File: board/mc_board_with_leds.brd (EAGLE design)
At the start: 131 x 76.6 mm, 30 parts, among them IC2 MEGA8-P, Q2 16MHz

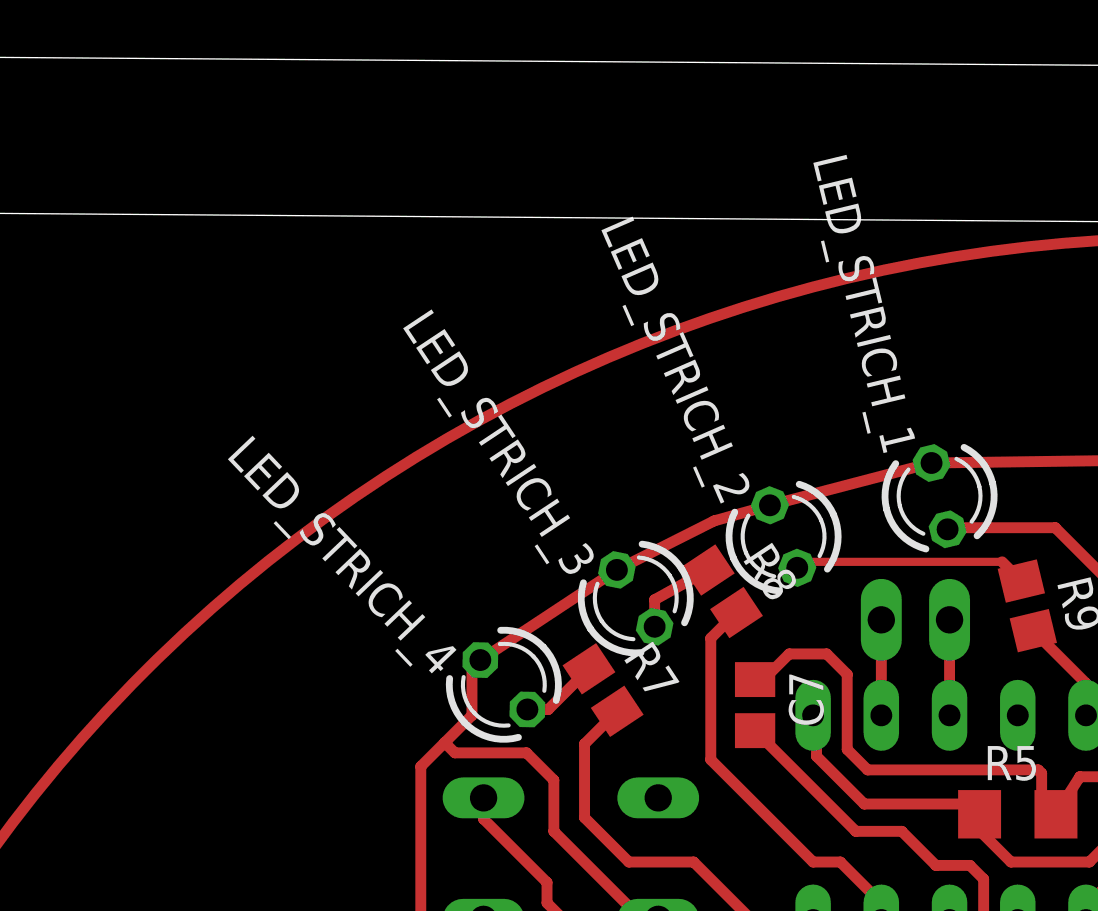
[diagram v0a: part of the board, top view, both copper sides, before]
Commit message: small changes
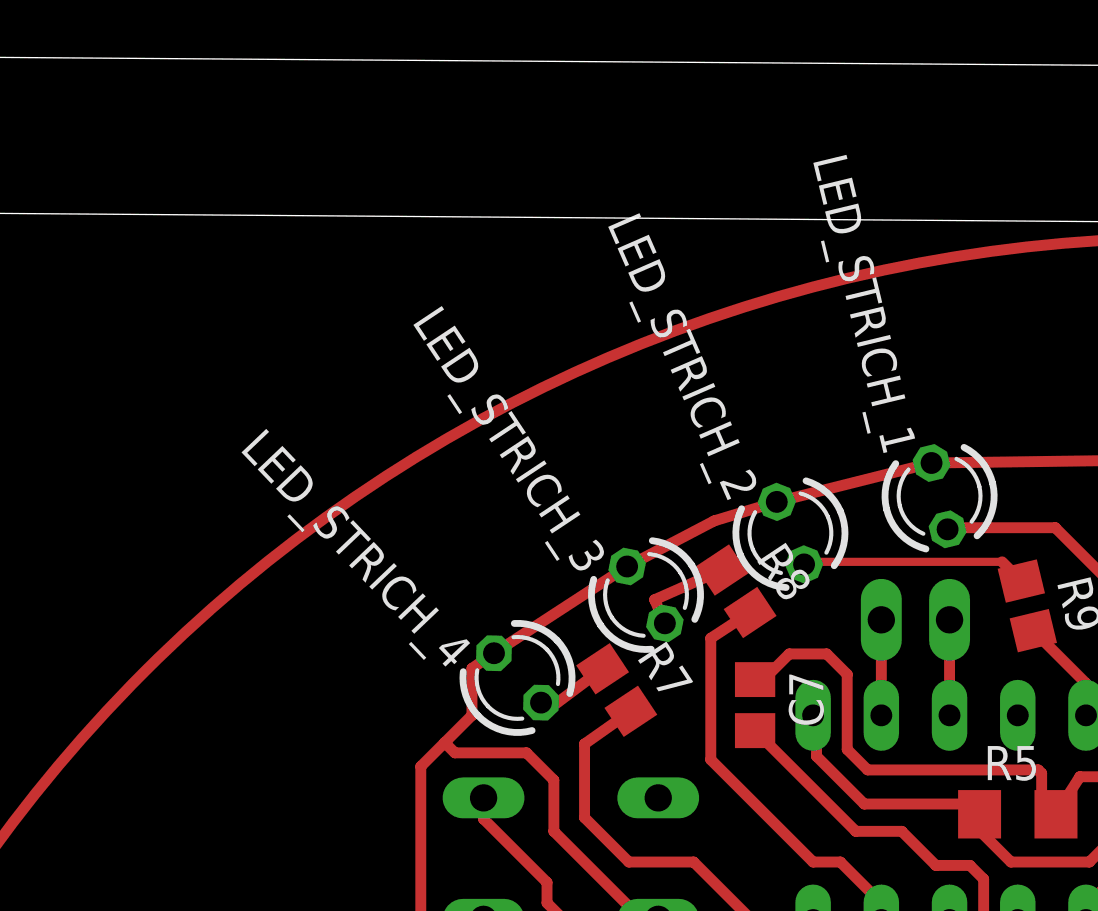
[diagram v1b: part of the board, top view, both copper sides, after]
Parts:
- moved LED_STRICH_4 0.57 mm to (30.1, 38.7)
- moved R7 0.51 mm to (33.8, 38.3)
- moved R8 0.51 mm to (38.3, 42.0)
- moved LED_STRICH_3 0.40 mm to (34.9, 41.8)
- moved LED_STRICH_2 0.28 mm to (40.3, 44.1)
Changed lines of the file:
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@@
 <element name="LED_ZAUN_2" library="led" package="LED3MM" value="" x="75.826471875" y="41.72945625" rot="R68.6"/>
 <element name="LED_ZAUN_1" library="led" package="LED3MM" value="" x="80.6571" y="38.7449125" rot="R58.6"/>
-<element name="LED_STRICH_4" library="led" package="LED3MM" value="" x="29.6350125" y="38.4763" rot="R133.6"/>
-<element name="LED_STRICH_3" library="led" package="LED3MM" value="" x="34.5460125" y="41.69431875" rot="R123.6"/>
-<element name="LED_STRICH_2" library="led" package="LED3MM" value="" x="40.04930625" y="43.994065625" rot="R113.6"/>
+<element name="LED_STRICH_4" library="led" package="LED3MM" value="" x="30.1430125" y="38.7303" rot="R133.6"/>
+<element name="LED_STRICH_3" library="led" package="LED3MM" value="" x="34.9270125" y="41.82131875" rot="R123.6"/>
+<element name="LED_STRICH_2" library="led" package="LED3MM" value="" x="40.30330625" y="44.121065625" rot="R113.6"/>
 <element name="LED_STRICH_1" library="led" package="LED3MM" value="" x="45.85698125" y="45.498234375" rot="R103.6"/>
 <element name="R1" library="resistor" package="R0805" value="470" x="67.091109375" y="41.668040625" rot="R258.6"/>
@@
 <element name="R4" library="resistor" package="R0805" value="470" x="77.496296875" y="38.99235" rot="R248.6"/>
 <element name="R6" library="resistor" package="R0805" value="470" x="83.281553125" y="34.931065625" rot="R138.6"/>
-<element name="R7" library="resistor" package="R0805" value="470" x="33.3296625" y="38.27971875" rot="R303.6"/>
-<element name="R8" library="resistor" package="R0805" value="470" x="37.7704875" y="41.957434375" rot="R303.6"/>
+<element name="R7" library="resistor" package="R0805" value="470" x="33.8376625" y="38.27971875" rot="R303.6"/>
+<element name="R8" library="resistor" package="R0805" value="470" x="38.2784875" y="41.957434375" rot="R303.6"/>
 <element name="R9" library="resistor" package="R0805" value="470" x="49.123534375" y="41.414296875" rot="R283.6"/>
 <element name="R10" library="resistor" package="R0805" value="470" x="53.788540625" y="40.819409375" rot="R269.6"/>
@@
 <wire x1="27.432" y1="36.322" x2="28.448" y2="37.338" width="0.4064" layer="1"/>
 <wire x1="28.448" y1="37.338" x2="28.448" y2="39.084803125" width="0.4064" layer="1"/>
-<wire x1="28.448" y1="39.084803125" x2="28.75919375" y2="39.395996875" width="0.4064" layer="1"/>
+<wire x1="28.448" y1="39.084803125" x2="29.26719375" y2="39.649996875" width="0.4064" layer="1"/>
 <wire x1="35.3822" y1="29.7434" x2="34.7726" y2="29.7434" width="0.4064" layer="1"/>
 <wire x1="34.7726" y1="29.7434" x2="31.496" y2="33.02" width="0.4064" layer="1"/>
@@
 <wire x1="59.555" y1="46.728" x2="59.42" y2="46.863" width="0.4064" layer="1"/>
 <wire x1="55.245" y1="46.863" x2="55.245" y2="46.085" width="0.4064" layer="1"/>
-<wire x1="45.55835" y1="46.732621875" x2="39.5408625" y2="45.15784375" width="0.4064" layer="1"/>
-<wire x1="39.5408625" y1="45.15784375" x2="37.465" y2="44.577" width="0.4064" layer="1"/>
-<wire x1="37.465" y1="44.577" x2="33.843203125" y2="42.752128125" width="0.4064" layer="1"/>
-<wire x1="33.843203125" y1="42.752128125" x2="28.75919375" y2="39.395996875" width="0.4064" layer="1"/>
+<wire x1="45.55835" y1="46.732621875" x2="39.7948625" y2="45.28484375" width="0.4064" layer="1"/>
+<wire x1="39.7948625" y1="45.28484375" x2="37.465" y2="44.577" width="0.4064" layer="1"/>
+<wire x1="37.465" y1="44.577" x2="34.224203125" y2="42.879128125" width="0.4064" layer="1"/>
+<wire x1="34.224203125" y1="42.879128125" x2="29.26719375" y2="39.649996875" width="0.4064" layer="1"/>
 <wire x1="55.245" y1="46.863" x2="45.55835" y2="46.732621875" width="0.4064" layer="1"/>
 <wire x1="55.245" y1="46.863" x2="59.555" y2="46.728" width="0.4064" layer="1"/>
@@
 <wire x1="34.29" y1="31.877" x2="32.639" y2="33.528" width="0.4064" layer="1"/>
 <wire x1="32.639" y1="33.528" x2="32.639" y2="36.27205625" width="0.4064" layer="1"/>
-<wire x1="32.639" y1="36.27205625" x2="33.855384375" y2="37.488440625" width="0.4064" layer="1"/>
+<wire x1="32.639" y1="36.27205625" x2="34.363384375" y2="37.488440625" width="0.4064" layer="1"/>
 </signal>
 <signal name="PC4/LED_STRICH_3">
@@
 <wire x1="41.148" y1="31.877" x2="37.338" y2="35.687" width="0.4064" layer="1"/>
 <wire x1="37.338" y1="35.687" x2="37.338" y2="40.207946875" width="0.4064" layer="1"/>
-<wire x1="37.338" y1="40.207946875" x2="38.296209375" y2="41.16615625" width="0.4064" layer="1"/>
+<wire x1="37.338" y1="40.207946875" x2="38.804209375" y2="41.16615625" width="0.4064" layer="1"/>
 </signal>
 <signal name="N$1">
@@
 <contactref element="R7" pad="1"/>
 <contactref element="LED_STRICH_4" pad="A"/>
-<wire x1="30.510828125" y1="37.5566" x2="31.28954375" y2="37.5566" width="0.4064" layer="1"/>
-<wire x1="31.28954375" y1="37.5566" x2="32.8039375" y2="39.07099375" width="0.4064" layer="1"/>
+<wire x1="31.018828125" y1="37.8106" x2="31.28954375" y2="37.5566" width="0.4064" layer="1"/>
+<wire x1="31.28954375" y1="37.5566" x2="33.3119375" y2="39.07099375" width="0.4064" layer="1"/>
 </signal>
 <signal name="N$10">
 <contactref element="R8" pad="1"/>
 <contactref element="LED_STRICH_3" pad="A"/>
-<wire x1="37.2447625" y1="42.748709375" x2="35.24881875" y2="41.641765625" width="0.4064" layer="1"/>
-<wire x1="35.24881875" y1="41.641765625" x2="35.24881875" y2="40.63650625" width="0.4064" layer="1"/>
+<wire x1="37.7527625" y1="42.748709375" x2="35.24881875" y2="41.641765625" width="0.4064" layer="1"/>
+<wire x1="35.24881875" y1="41.641765625" x2="35.62981875" y2="40.76350625" width="0.4064" layer="1"/>
 </signal>
 <signal name="N$11">
@@
 <wire x1="48.900146875" y1="42.337659375" x2="48.18480625" y2="43.053" width="0.4064" layer="1"/>
 <wire x1="48.18480625" y1="43.053" x2="40.7804625" y2="43.053" width="0.3048" layer="1"/>
-<wire x1="40.557746875" y1="42.830284375" x2="40.7804625" y2="43.053" width="0.4064" layer="1"/>
+<wire x1="40.811746875" y1="42.957284375" x2="40.7804625" y2="43.053" width="0.4064" layer="1"/>
 </signal>
 <signal name="N$12">
